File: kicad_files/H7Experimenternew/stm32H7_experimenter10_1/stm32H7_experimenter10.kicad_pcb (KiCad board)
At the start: 4 copper layers, 63.2 x 86.1 mm, 79 parts, among them IC1 AD8659, IC2 7805TV, IC3 AD8659, IC5 6N138, P1 RK09SONGHUEI, P2 RK09SONGHUEI, P3 RK09SONGHUEI, P4 RK09SONGHUEI, P5 RK09SONGHUEI, P6 RK09SONGHUEI

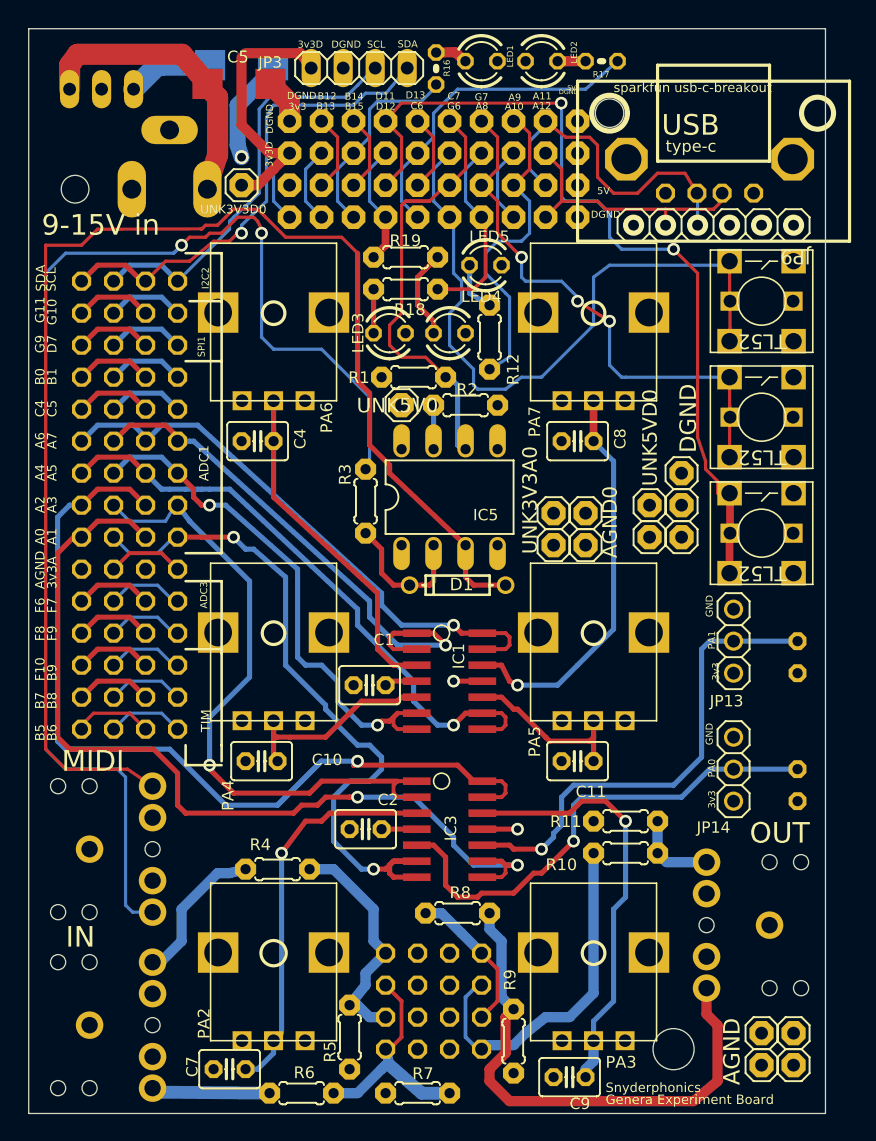
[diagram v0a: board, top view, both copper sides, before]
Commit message: experimenter kicad
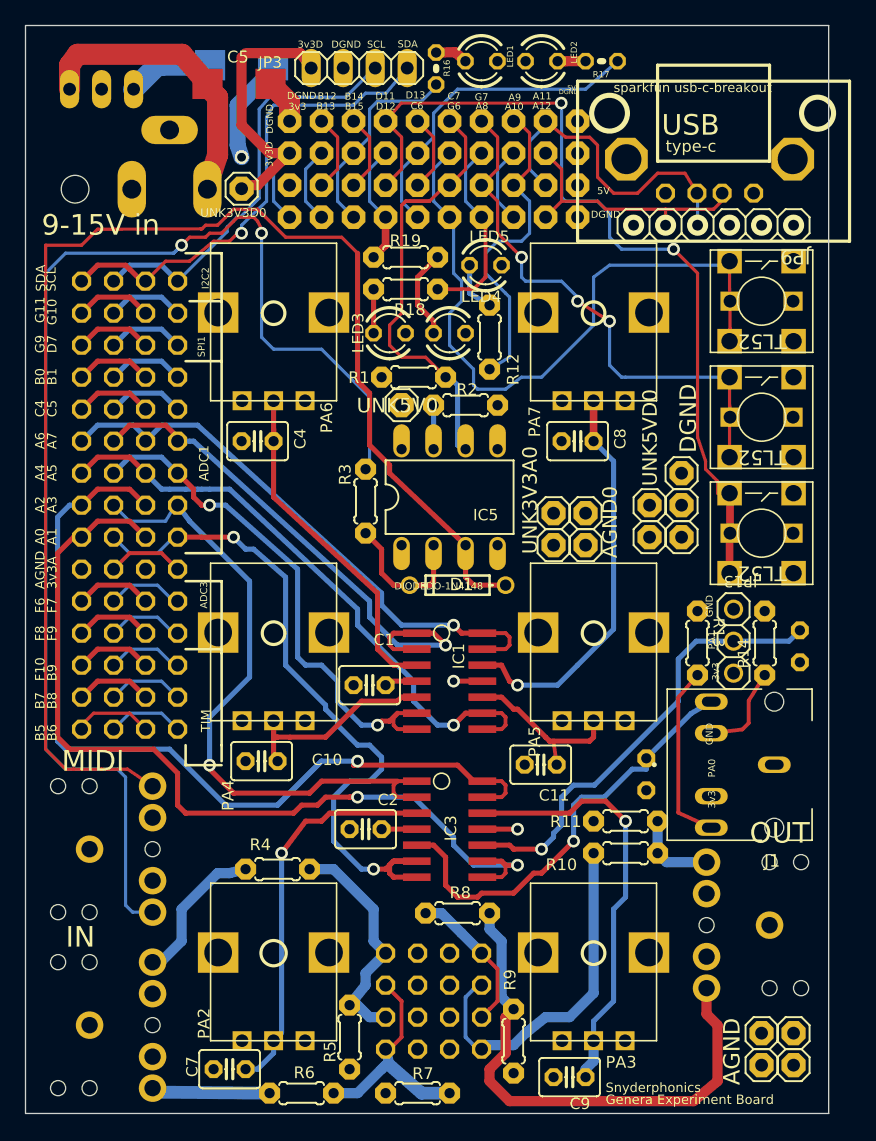
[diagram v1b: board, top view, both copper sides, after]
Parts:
- removed JP14: , stm32H7_experimenter10:1X03
- removed UNK_HOLE_0: , stm32H7_experimenter10:dummyfp0
- removed UNK_HOLE_1: , stm32H7_experimenter10:dummyfp1
- added J1: SJ1-3555NG, Snapeda:CUI_SJ1-3555NG, F.Cu at (176.0, 119.9)
- added R13: 220R, stm32H7_experimenter10:0204_5, F.Cu at (169.9, 110.2)
- added R14: 10k, stm32H7_experimenter10:0204_5, F.Cu at (175.3, 110.2)
- AGND0, AGND1, AGND2, AGND3, AGND4, AGND5, DGND1, DGND2, DGND3, UNK3V3A0, UNK3V3A1, UNK3V3D0, UNK5V0, UNK5V2, UNK5VD0: value (none) -> PINHD-1X1
- D1: value (none) -> DIODEDO-1N4148
- IC2: value 7805TV -> 78TV
- JP1, JP2: value (none) -> PINHD-2X10
- JP10, JP7, JP8: value (none) -> AUDIO-JACKPTH
- JP12, JP6: value (none) -> PINHD-2X4
- JP13: value (none) -> PINHD-1X3
- JP3: value (none) -> PINHD-1X4
- JP4, JP5: value (none) -> PINHD-2X15
- JP9: value (none) -> PINHD-1X6
- LED1, LED2, LED3, LED4, LED5: value (none) -> LED3MM
- moved C16 12.0 mm to (165.9, 120.7)
- moved C11 2.94 mm to (157.5, 119.9)
- moved C17 0.88 mm to (178.1, 110.5)
- moved UNK3V3D0 0.28 mm to (133.7, 74.2)
- turned JP13 to -90 degrees
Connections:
- net 3V3A renamed 3V3
- net 3V3D renamed /3V3D
- net PA0 renamed /PA0
- net PA1 renamed /PA1
- net PA10 renamed /PA10
- net PA11 renamed /PA11
- net PA12 renamed /PA12
- net PA2 renamed /PA2
- net PA3 renamed /PA3
- net PA4 renamed /PA4
- net PA5 renamed /PA5
- net PA6 renamed /PA6
- net PA7 renamed /PA7
- net PA8 renamed /PA8
- net PA9 renamed /PA9
- net PB0 renamed /PB0
- net PB1 renamed /PB1
- net PB12 renamed /PB12
- net PB13 renamed /PB13
- net PB14 renamed /PB14
- net PB15 renamed /PB15
- net PC4 renamed /PC4
- net PC5 renamed /PC5
- net PC6 renamed /PC6
- net PC7 renamed /PC7
- net PD11 renamed /PD11
- net PD12 renamed /PD12
- net PD13 renamed /PD13
- net PG6 renamed /PG6
- net PG7 renamed /PG7
- net SCL renamed /SCL
- net SDA renamed /SDA
- JP10 pad SLEEVE: (no net) -> unconnected-(JP10-PadSLEEVE)
- JP9 pad 3: (no net) -> unconnected-(JP9-Pad3)
- JP9 pad 6: (no net) -> unconnected-(JP9-Pad6)
- U$1 pad 3: (no net) -> unconnected-(U$1-Pad3)
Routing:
- net DGND: track 64.5 -> 102.7 mm
- net (no net): track 0.00 -> 31.8 mm
- net N$30: track 15.9 -> 0.00 mm
- net N$29: track 15.9 -> 0.00 mm
- net Net-(J1-Pad3): track 0.00 -> 14.4 mm
- net Net-(J1-Pad4): track 0.00 -> 7.37 mm
- net Net-(IC3-+INB): track 39.1 -> 34.9 mm
- net Net-(IC3-+INC): track 38.5 -> 36.0 mm
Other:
- board size 63.2 x 86.1 mm -> 63.8 x 86.4 mm
